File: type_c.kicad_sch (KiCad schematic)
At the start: 14 parts, among them U12 FUSB302B, U14 DPO2036

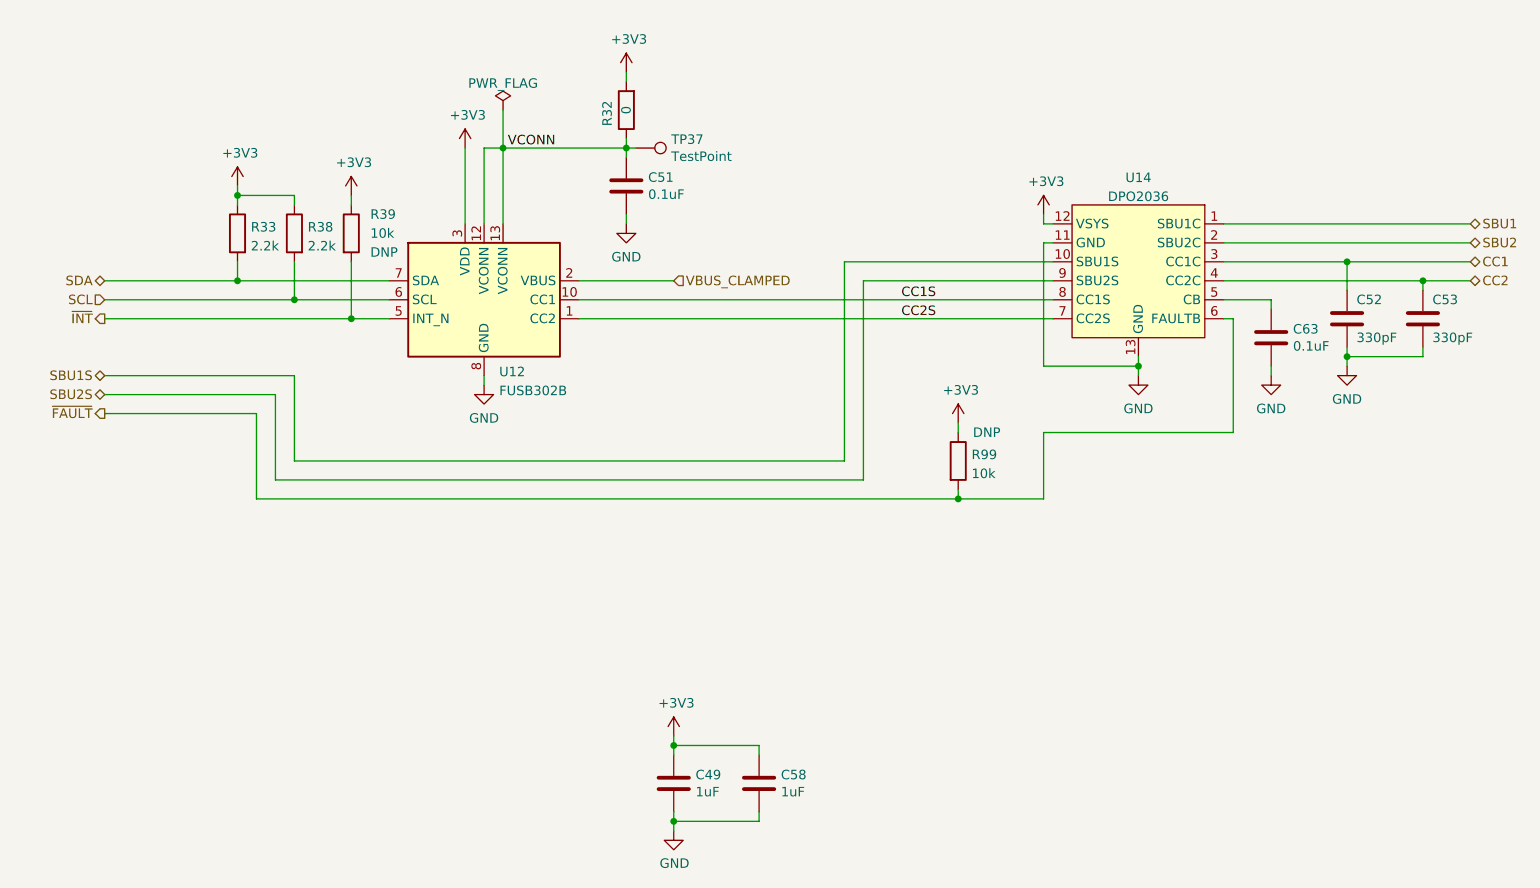
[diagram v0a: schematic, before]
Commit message: Add files via upload
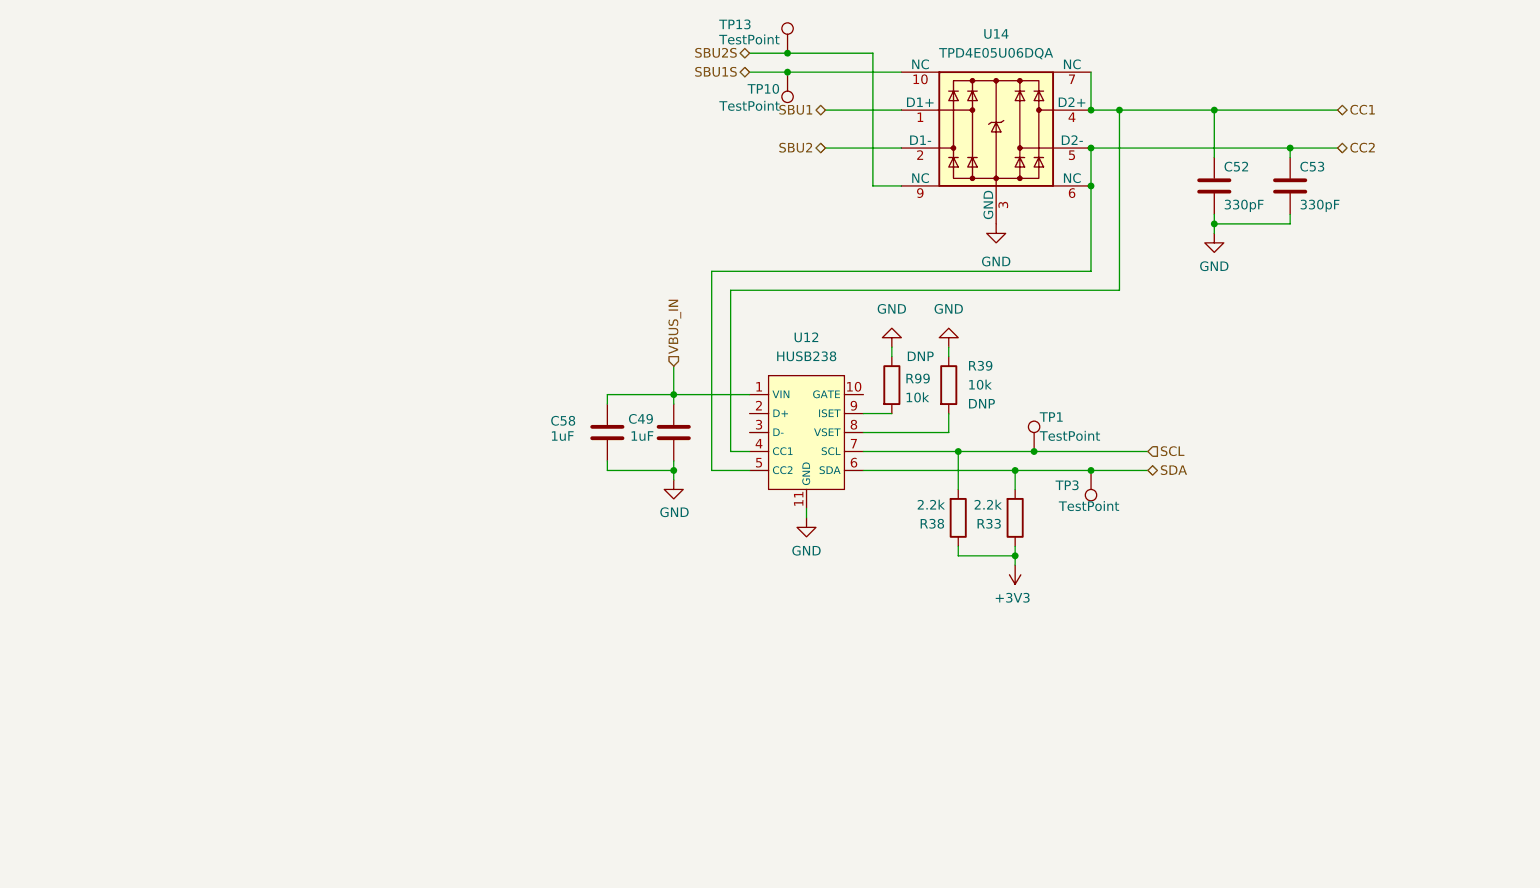
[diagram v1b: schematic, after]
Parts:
- removed C51, C63: 0.1uF, Capacitor_SMD:C_0402_1005Metric, symbol Device:C
- removed R32: 0, Resistor_SMD:R_0402_1005Metric, symbol Device:R
- removed TP37: TestPoint, TestPoint:TestPoint_Pad_D1.0mm, symbol Connector:TestPoint
- removed U12: FUSB302B, Package_DFN_QFN:WQFN-14-1EP_2.5x2.5mm_P0.5mm_EP1.45x1.45mm, symbol Interface_USB:FUSB302BMPX
- removed U14: DPO2036, cynthion:Diodes_UQFN2020-12_Type-B, symbol usb:DPO2036
- added TP1, TP10, TP13, TP3: TestPoint, TestPoint:TestPoint_Pad_D1.0mm, symbol Connector:TestPoint
- added U12: HUSB238, Porject:HUSB238-QFN-10_EP_3.7x3_Pitch0.5mm, symbol Project:HUSB238
- added U14: TPD4E05U06DQA, Package_SON:USON-10_2.5x1.0mm_P0.5mm, symbol Power_Protection:TPD4E05U06DQA
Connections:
- net +3V3: no longer C49.1, C58.1, R39.1, R99.1
- net CC1: now also U12.4 (CC1), U14.4 (D2+), U14.7 (NC)
- net CC2: now also U12.5 (CC2), U14.5 (D2-), U14.6 (NC)
- net GND: now also R39.1, R99.1, U12.11 (GND), U14.3 (GND), U14.8 (GND)
- net SBU1: now also U14.1 (D1+)
- net SBU1S: now also TP10.1, U14.10 (NC)
- net SBU2: now also U14.2 (D1-)
- net SBU2S: now also TP13.1, U14.9 (NC)
- net SCL: now also TP1.1, U12.7 (SCL)
- net SDA: now also TP3.1, U12.6 (SDA)
- net ~{FAULT}: no longer names the net of R99.2
- net ~{FAULT}: now also U12.9 (ISET)
- net ~{INT}: no longer names the net of R39.2
- net ~{INT}: now also U12.8 (VSET)
- new net VBUS_IN: C49.1, C58.1, U12.1 (VIN)
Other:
- moved on the sheet: C49, C52, C53, C58, R33, R38, R39, R99
